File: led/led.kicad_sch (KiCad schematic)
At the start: 8 parts, among them J1 Screw_Terminal_01x10, J2 Screw_Terminal_01x03, J3 Screw_Terminal_01x01

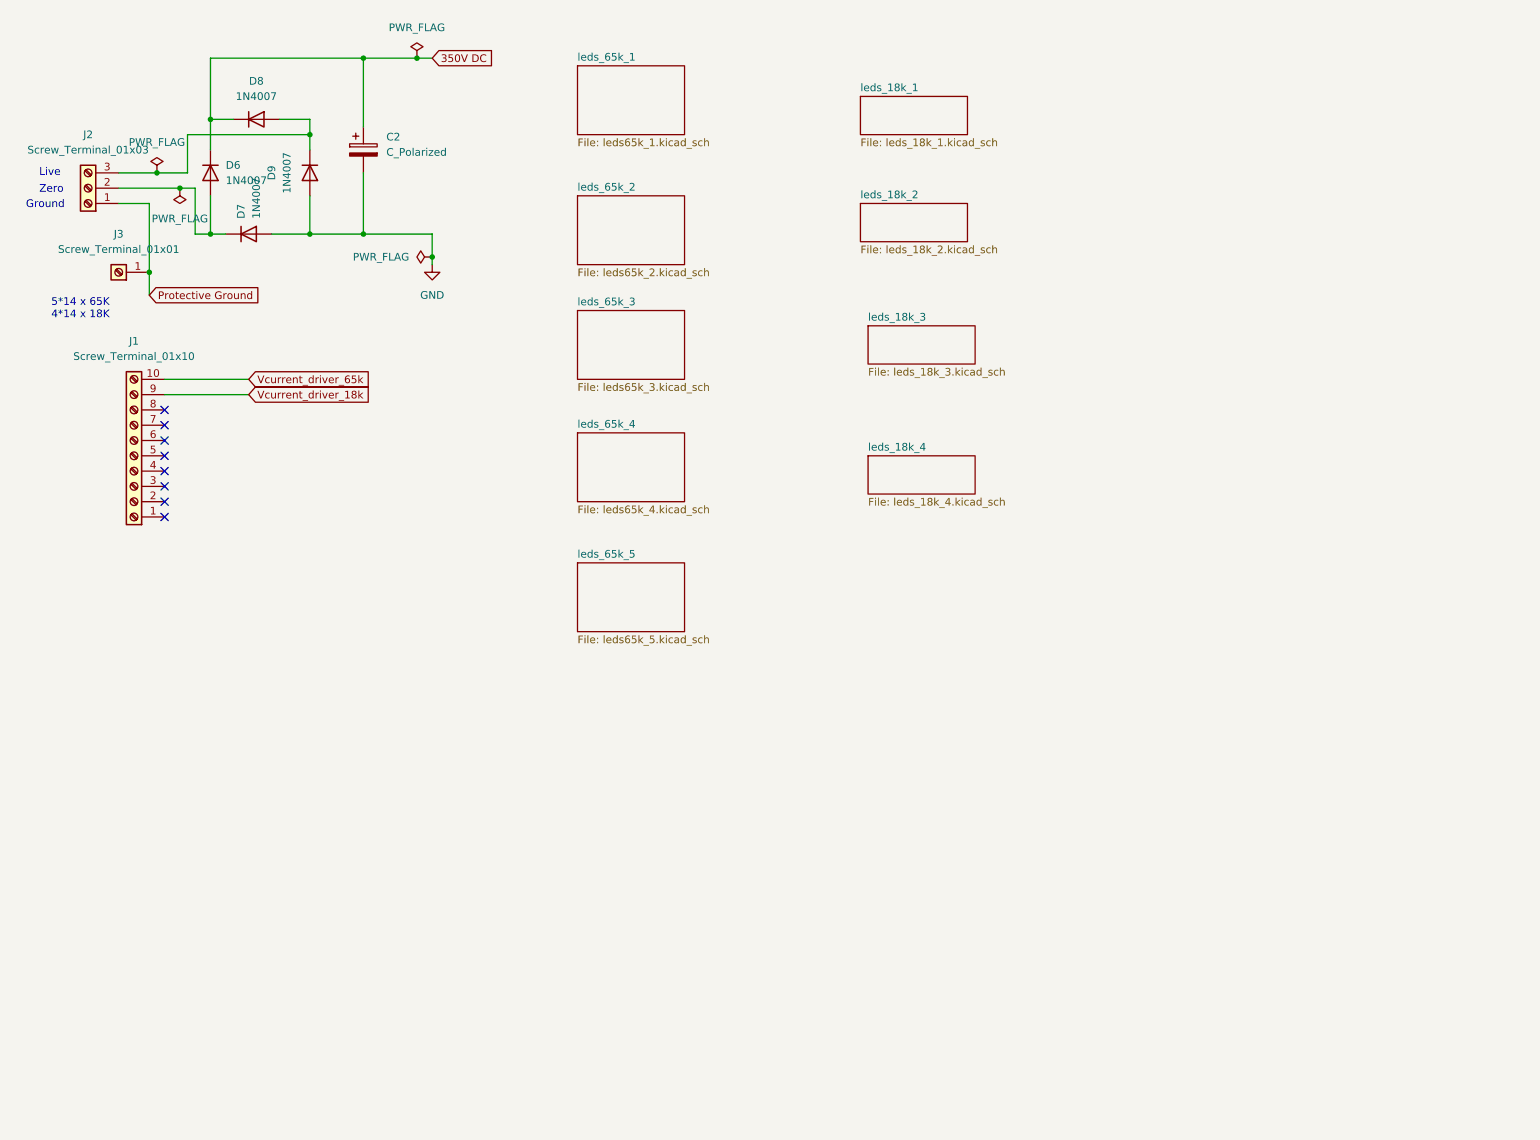
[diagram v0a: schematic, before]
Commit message: schematics with 5050 leds ready
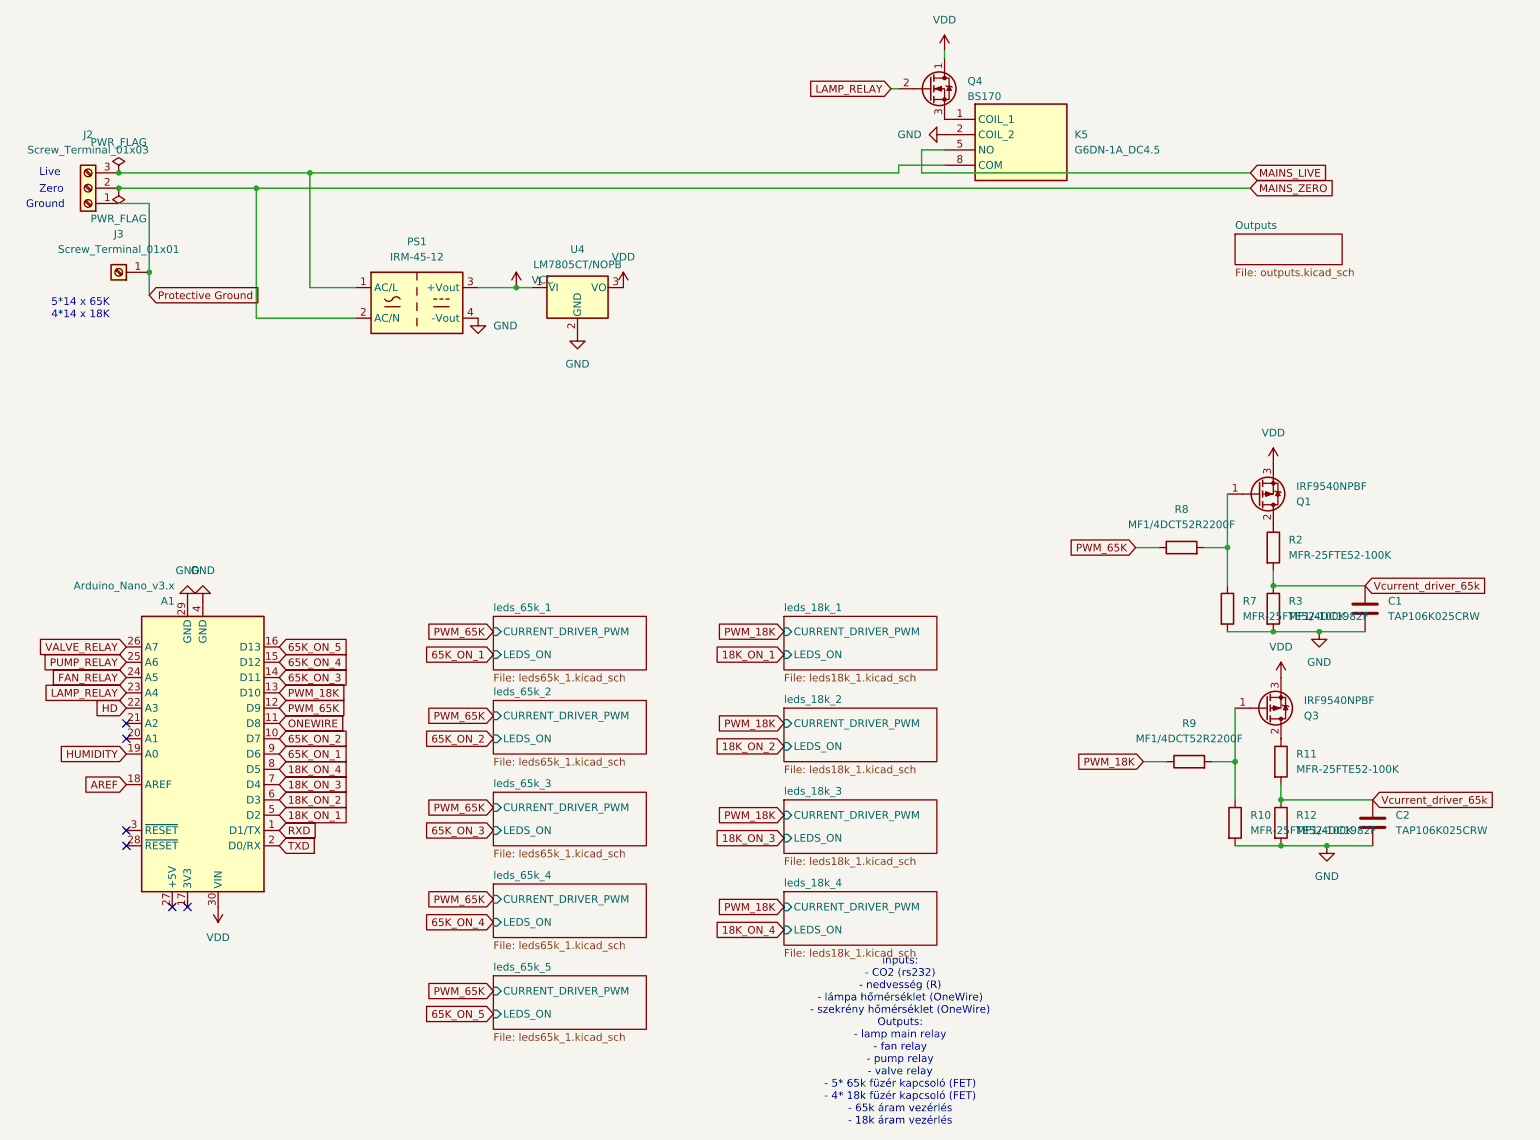
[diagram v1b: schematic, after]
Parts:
- removed C2: C_Polarized, symbol Device:C_Polarized
- removed D6, D7, D8, D9: 1N4007, Diode_THT:D_DO-41_SOD81_P10.16mm_Horizontal, symbol Diode:1N4007
- removed J1: Screw_Terminal_01x10, symbol Connector:Screw_Terminal_01x10
- added A1: Arduino_Nano_v3.x, Module:Arduino_Nano, symbol MCU_Module:Arduino_Nano_v3.x
- added C1, C2: TAP106K025CRW, Resistor_THT:R_Axial_DIN0204_L3.6mm_D1.6mm_P2.54mm_Vertical, symbol Device:C
- added K5: G6DN-1A_DC4.5, arduino-library:G6DN1ADC45, symbol G6DN-1A_DC4_5:G6DN-1A_DC4.5
- added PS1: IRM-45-12, arduino-library:IRM-45, symbol Converter_ACDC:IRM-60-12
- added Q1, Q3: IRF9540NPBF, Package_TO_SOT_THT:TO-220-3_Vertical, symbol Transistor_FET:IRF9540N
- added Q4: BS170, Package_TO_SOT_THT:TO-92_Inline, symbol Transistor_FET:BS170
- added R10, R11, R2, R7: MFR-25FTE52-100K, Resistor_THT:R_Axial_DIN0204_L3.6mm_D1.6mm_P2.54mm_Vertical, symbol Device:R
- added R12, R3: MF1/4DC1982F, Resistor_THT:R_Axial_DIN0204_L3.6mm_D1.6mm_P2.54mm_Vertical, symbol Device:R
- added R8, R9: MF1/4DCT52R2200F, Resistor_THT:R_Axial_DIN0204_L3.6mm_D1.6mm_P2.54mm_Vertical, symbol Device:R
- added U4: LM7805CT/NOPB, Package_TO_SOT_THT:TO-220-3_Vertical, symbol Regulator_Linear:LM7805_TO220
- J2: footprint (none) -> Connector_Wire:SolderWire-1.5sqmm_1x03_P6mm_D1.7mm_OD3mm; now left out of the parts list
- J3: footprint (none) -> Connector_Wire:SolderWire-1.5sqmm_1x01_D1.7mm_OD3.9mm; now left out of the parts list
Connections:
- net GND: now also A1.29 (GND), A1.4 (GND), C1.2, C2.2, K5.2 (COIL_2), PS1.4 (-Vout), R10.2, R12.2, R3.2, R7.2, U4.2 (GND)
- net Vcurrent_driver_65k: now also C1.1, C2.1, R11.2, R12.1, R2.2, R3.1
- net MAINS_ZERO: now reaches J2.2 (Pin_2)
- net MAINS_ZERO: now also PS1.2 (AC/N)
- net at J2.3 (Pin_3): now also K5.8 (COM), PS1.1 (AC/L)
- new net: Q3.2 (D), R11.1
- new net: Q3.1 (G), R10.1, R9.2
- new net: K5.1 (COIL_1), Q4.3 (S)
- new net: Q1.1 (G), R7.1, R8.2
- new net: Q1.2 (D), R2.1
- new net 18K_ON_1: A1.5 (D2)
- new net 18K_ON_2: A1.6 (D3)
- new net 18K_ON_3: A1.7 (D4)
- new net 18K_ON_4: A1.8 (D5)
- new net 65K_ON_1: A1.9 (D6)
- new net 65K_ON_2: A1.10 (D7)
- new net 65K_ON_3: A1.14 (D11)
- new net 65K_ON_4: A1.15 (D12)
- new net 65K_ON_5: A1.16 (D13)
- new net AREF: A1.18 (AREF)
- new net FAN_RELAY: A1.24 (A5)
- new net HD: A1.22 (A3)
- new net HUMIDITY: A1.19 (A0)
- new net LAMP_RELAY: A1.23 (A4), Q4.2 (G)
- new net MAINS_LIVE: K5.5 (NO)
- new net ONEWIRE: A1.11 (D8)
- new net PUMP_RELAY: A1.25 (A6)
- new net PWM_18K: A1.13 (D10), R9.1
- new net PWM_65K: A1.12 (D9), R8.1
- new net RXD: A1.1 (D1/TX)
- new net TXD: A1.2 (D0/RX)
- new net VALVE_RELAY: A1.26 (A7)
- new net VCC: PS1.3 (+Vout), U4.1 (VI)
- new net VDD: A1.30 (VIN), Q1.3 (S), Q3.3 (S), Q4.1 (D), U4.3 (VO)
- no-connect marks 8 -> 6
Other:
- added sheet Outputs (outputs.kicad_sch)
- sheet leds_18k_1: file leds_18k_1.kicad_sch -> leds18k_1.kicad_sch
- sheet leds_18k_1 ports: added CURRENT_DRIVER_PWM, LEDS_ON; removed none
- sheet leds_18k_2: file leds_18k_2.kicad_sch -> leds18k_1.kicad_sch
- sheet leds_18k_2 ports: added CURRENT_DRIVER_PWM, LEDS_ON; removed none
- sheet leds_18k_3: file leds_18k_3.kicad_sch -> leds18k_1.kicad_sch
- sheet leds_18k_3 ports: added CURRENT_DRIVER_PWM, LEDS_ON; removed none
- sheet leds_18k_4: file leds_18k_4.kicad_sch -> leds18k_1.kicad_sch
- sheet leds_18k_4 ports: added CURRENT_DRIVER_PWM, LEDS_ON; removed none
- sheet leds_65k_1 ports: added CURRENT_DRIVER_PWM, LEDS_ON; removed none
- sheet leds_65k_2: file leds65k_2.kicad_sch -> leds65k_1.kicad_sch
- sheet leds_65k_2 ports: added CURRENT_DRIVER_PWM, LEDS_ON; removed none
- sheet leds_65k_3: file leds65k_3.kicad_sch -> leds65k_1.kicad_sch
- sheet leds_65k_3 ports: added CURRENT_DRIVER_PWM, LEDS_ON; removed none
- sheet leds_65k_4: file leds65k_4.kicad_sch -> leds65k_1.kicad_sch
- sheet leds_65k_4 ports: added CURRENT_DRIVER_PWM, LEDS_ON; removed none
- sheet leds_65k_5: file leds65k_5.kicad_sch -> leds65k_1.kicad_sch
- sheet leds_65k_5 ports: added CURRENT_DRIVER_PWM, LEDS_ON; removed none
- note added: "inputs: - CO2 (rs232) - nedvesség (R) - lámpa hőmérséklet (OneWire) - szekrény hőmérséklet (OneWire) Outputs: - lamp main relay - fan relay - pump relay - valve relay - 5* 65k füzér kapcsoló (FET) - 4* 18k füzér kapcsoló (FET) - 65k áram vezérlés - 18k áram vezérlés"
